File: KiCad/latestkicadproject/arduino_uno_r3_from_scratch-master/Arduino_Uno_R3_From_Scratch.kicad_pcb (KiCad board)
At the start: 2 copper layers, 50.8 x 58.4 mm, 36 parts, among them IC1 MC33269ST-5.OT3, IC5 ATMEGA328P-MU, P1 CONN_01X06, P2 IOH, P3 AD, P4 H4, SW1 RESET_SWITCH, U2 LP2985-33DBVR, U3 74AHC1G04, U4 74AHC1G04, U9 L298, X1 DG3XX-04-3.5, X2 DG3XX-02-3.5, Y2 Crystal

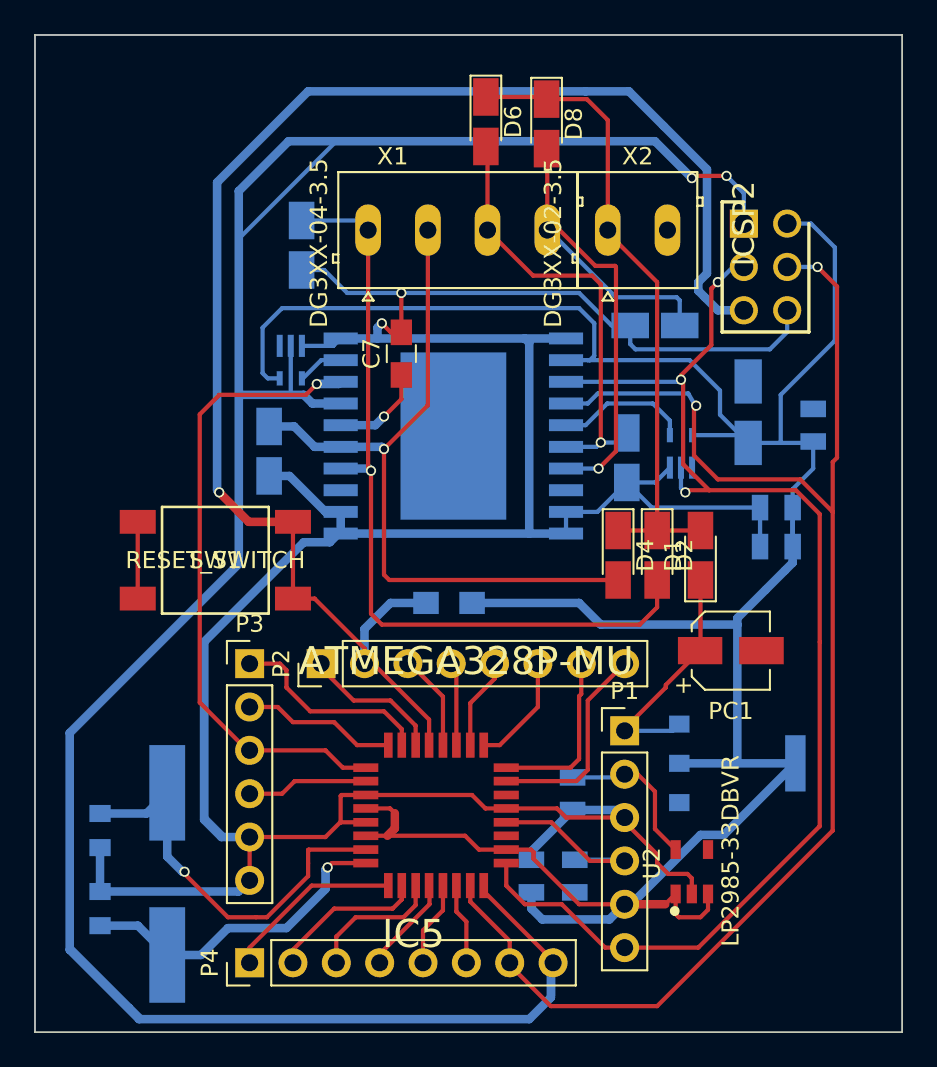
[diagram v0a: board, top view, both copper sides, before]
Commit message: PCB routing v1
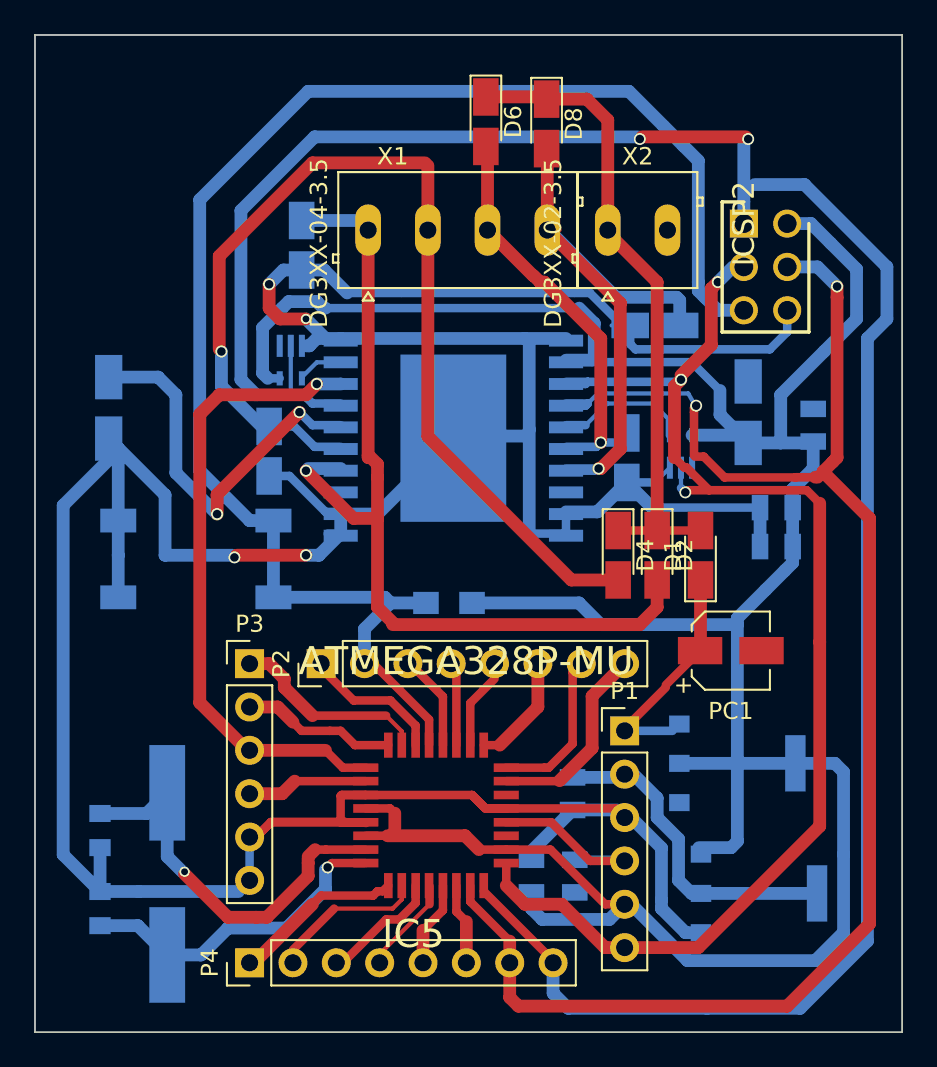
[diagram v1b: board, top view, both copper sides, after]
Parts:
- removed U2: LP2985-33DBVR, LP2985-33DBVR:SOT95P280X145-5N
- removed U9: L298, L298P:SOIC127P1420X360-21N
- added IC2: MC33269ST-5.OT3, MC33269ST-3.3T3G:SOT230P700X175-4N, B.Cu at (100.6, 105.8)
- added IC3: L298P, L298Poud:SOIC127P1420X360-21N, B.Cu at (82.7, 79.1)
- C7: footprint Capacitors_SMD:C_0805_HandSoldering -> Capacitors_SMD:CP_Elec_4x5.3; moved to B.Cu
- SW1: moved to B.Cu
- moved C7 17.4 mm to (62.5, 77.3), turned to 270 degrees
- moved SW1 4.71 mm to (72.1, 83.9)
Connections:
- ICSP2 pad 6: GND -> Net-(ICSP2-Pad6)
- SW1 pad 1: Net-(SW1-Pad1) -> GND
- SW1 pad 2: Net-(SW1-Pad1) -> GND
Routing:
- net /ATMEGA328P/DIRA: track 235.0 -> 135.5 mm
- net +5V: track 157.3 -> 181.8 mm
- net GND: track 239.0 -> 263.4 mm, vias 2 -> 4
- net /Driver/OUT2: track 45.8 -> 62.7 mm
- net /Driver/PWRIN: track 6.32 -> 23.1 mm, vias 1 -> 2
- net /Headers/+3V3: track 9.22 -> 20.1 mm
- net /ATMEGA328P/PWMB: track 85.9 -> 95.9 mm
- net /Driver/OUT1: track 47.7 -> 53.2 mm
- net Net-(SW1-Pad1): track 4.50 -> 0.00 mm
- net /ATMEGA328P/DIRB: track 74.9 -> 77.0 mm
- net /Driver/OUT4: track 34.6 -> 36.5 mm
- net /Driver/OUT3: track 26.1 -> 24.2 mm
- net /ATMEGA328P/PWMA: track 38.7 -> 37.4 mm
- net Net-(ICSP2-Pad6): track 0.00 -> 1.27 mm
- net /ATMEGA328P/IO7: track 8.09 -> 7.12 mm
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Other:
- net class 0.5: via_dia 0.6 -> 0.7; via_drill 0.4 -> 0.5
- net class 30mills added: clearance 0.25, trace_width 0.75, via_dia 0.7, via_drill 0.5
- net class 40mills: clearance 1.016 -> 0.25; trace_width 1.016 -> 1
